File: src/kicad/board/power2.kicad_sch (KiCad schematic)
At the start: 22 parts, among them J6 PWR_EN, Q1 DMG2305UX, U2 BQ25172, U3 TLV61070A, U4 XC6206P332MR

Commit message: wip
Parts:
- C4, C5, C7, C8, C9: footprint Capacitor_SMD:C_0805_2012Metric -> Capacitor_SMD:C_0603_1608Metric; Vendor C15850 -> C19702
- C6: footprint Capacitor_SMD:C_0805_2012Metric -> Capacitor_SMD:C_0603_1608Metric; Vendor C45783 -> C59461
- R13, R15: footprint Resistor_SMD:R_0805_2012Metric -> Resistor_SMD:R_0603_1608Metric; Vendor C17530 -> C13167
- R16: footprint Resistor_SMD:R_0805_2012Metric -> Resistor_SMD:R_0603_1608Metric; Vendor C17593 -> C22967
- R17: footprint Resistor_SMD:R_0805_2012Metric -> Resistor_SMD:R_0603_1608Metric; Vendor C4328 -> C4184
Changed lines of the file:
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@@
       (effects (font (size 1.27 1.27)) (justify left))
     )
-    (property "Footprint" "Capacitor_SMD:C_0805_2012Metric" (id 2) (at 199.0852 140.97 0)
+    (property "Footprint" "Capacitor_SMD:C_0603_1608Metric" (id 2) (at 199.0852 140.97 0)
       (effects (font (size 1.27 1.27)) hide)
     )
@@
       (effects (font (size 1.27 1.27)) hide)
     )
-    (property "Vendor" "C15850" (id 4) (at 198.12 137.16 0)
+    (property "Vendor" "C19702" (id 4) (at 198.12 137.16 0)
       (effects (font (size 1.27 1.27)) hide)
     )
@@
       (effects (font (size 1.27 1.27)) (justify left))
     )
-    (property "Footprint" "Capacitor_SMD:C_0805_2012Metric" (id 2) (at 121.6152 109.22 0)
+    (property "Footprint" "Capacitor_SMD:C_0603_1608Metric" (id 2) (at 121.6152 109.22 0)
       (effects (font (size 1.27 1.27)) hide)
     )
@@
       (effects (font (size 1.27 1.27)) hide)
     )
-    (property "Vendor" "C15850" (id 4) (at 120.65 105.41 0)
+    (property "Vendor" "C19702" (id 4) (at 120.65 105.41 0)
       (effects (font (size 1.27 1.27)) hide)
     )
@@
       (effects (font (size 1.27 1.27)) (justify left))
     )
-    (property "Footprint" "Resistor_SMD:R_0805_2012Metric" (id 2) (at 159.512 66.04 90)
+    (property "Footprint" "Resistor_SMD:R_0603_1608Metric" (id 2) (at 159.512 66.04 90)
       (effects (font (size 1.27 1.27)) hide)
     )
@@
       (effects (font (size 1.27 1.27)) hide)
     )
-    (property "Vendor" "C4328" (id 4) (at 161.29 66.04 0)
+    (property "Vendor" "C4184" (id 4) (at 161.29 66.04 0)
       (effects (font (size 1.27 1.27)) hide)
     )
@@
       (effects (font (size 1.27 1.27)) (justify left))
     )
-    (property "Footprint" "Resistor_SMD:R_0805_2012Metric" (id 2) (at 151.257 133.35 90)
+    (property "Footprint" "Resistor_SMD:R_0603_1608Metric" (id 2) (at 151.257 133.35 90)
       (effects (font (size 1.27 1.27)) hide)
     )
@@
       (effects (font (size 1.27 1.27)) hide)
     )
-    (property "Vendor" "C17530" (id 4) (at 153.035 133.35 0)
+    (property "Vendor" "C13167" (id 4) (at 153.035 133.35 0)
       (effects (font (size 1.27 1.27)) hide)
     )
@@
     (property "Reference" "R13" (id 0) (at 132.08 43.18 90))
     (property "Value" "2K7" (id 1) (at 132.08 45.72 90))
-    (property "Footprint" "Resistor_SMD:R_0805_2012Metric" (id 2) (at 132.08 47.498 90)
+    (property "Footprint" "Resistor_SMD:R_0603_1608Metric" (id 2) (at 132.08 47.498 90)
       (effects (font (size 1.27 1.27)) hide)
     )
@@
       (effects (font (size 1.27 1.27)) hide)
     )
-    (property "Vendor" "C17530" (id 4) (at 132.08 45.72 0)
+    (property "Vendor" "C13167" (id 4) (at 132.08 45.72 0)
       (effects (font (size 1.27 1.27)) hide)
     )
@@
       (effects (font (size 1.27 1.27)) (justify left))
     )
-    (property "Footprint" "Capacitor_SMD:C_0805_2012Metric" (id 2) (at 169.8752 69.85 0)
+    (property "Footprint" "Capacitor_SMD:C_0603_1608Metric" (id 2) (at 169.8752 69.85 0)
       (effects (font (size 1.27 1.27)) hide)
     )
@@
       (effects (font (size 1.27 1.27)) hide)
     )
-    (property "Vendor" "C15850" (id 4) (at 168.91 66.04 0)
+    (property "Vendor" "C19702" (id 4) (at 168.91 66.04 0)
       (effects (font (size 1.27 1.27)) hide)
     )
@@
       (effects (font (size 1.27 1.27)) (justify left))
     )
-    (property "Footprint" "Capacitor_SMD:C_0805_2012Metric" (id 2) (at 176.2252 140.97 0)
+    (property "Footprint" "Capacitor_SMD:C_0603_1608Metric" (id 2) (at 176.2252 140.97 0)
       (effects (font (size 1.27 1.27)) hide)
     )
@@
       (effects (font (size 1.27 1.27)) hide)
     )
-    (property "Vendor" "C15850" (id 4) (at 175.26 137.16 0)
+    (property "Vendor" "C19702" (id 4) (at 175.26 137.16 0)
       (effects (font (size 1.27 1.27)) hide)
     )
@@
       (effects (font (size 1.27 1.27)) (justify left))
     )
-    (property "Footprint" "Resistor_SMD:R_0805_2012Metric" (id 2) (at 153.162 66.04 90)
+    (property "Footprint" "Resistor_SMD:R_0603_1608Metric" (id 2) (at 153.162 66.04 90)
       (effects (font (size 1.27 1.27)) hide)
     )
@@
       (effects (font (size 1.27 1.27)) hide)
     )
-    (property "Vendor" "C17593" (id 4) (at 154.94 66.04 0)
+    (property "Vendor" "C22967" (id 4) (at 154.94 66.04 0)
       (effects (font (size 1.27 1.27)) hide)
     )
@@
       (effects (font (size 1.27 1.27)) (justify left))
     )
-    (property "Footprint" "Capacitor_SMD:C_0805_2012Metric" (id 2) (at 108.9152 66.04 0)
+    (property "Footprint" "Capacitor_SMD:C_0603_1608Metric" (id 2) (at 108.9152 66.04 0)
       (effects (font (size 1.27 1.27)) hide)
     )
@@
       (effects (font (size 1.27 1.27)) hide)
     )
-    (property "Vendor" "C15850" (id 4) (at 107.95 62.23 0)
+    (property "Vendor" "C19702" (id 4) (at 107.95 62.23 0)
       (effects (font (size 1.27 1.27)) hide)
     )
@@
       (effects (font (size 1.27 1.27)) (justify left))
     )
-    (property "Footprint" "Capacitor_SMD:C_0805_2012Metric" (id 2) (at 164.1602 128.27 0)
+    (property "Footprint" "Capacitor_SMD:C_0603_1608Metric" (id 2) (at 164.1602 128.27 0)
       (effects (font (size 1.27 1.27)) hide)
     )
@@
       (effects (font (size 1.27 1.27)) hide)
     )
-    (property "Vendor" "C45783" (id 4) (at 163.195 124.46 0)
-      (effects (font (size 1.27 1.27)) hide)
-    )
+    (property "Vendor" "C59461" (id 4) (at 163.195 124.46 0)
+      (effects (font (size 1.27 1.27)) hide)
+    )

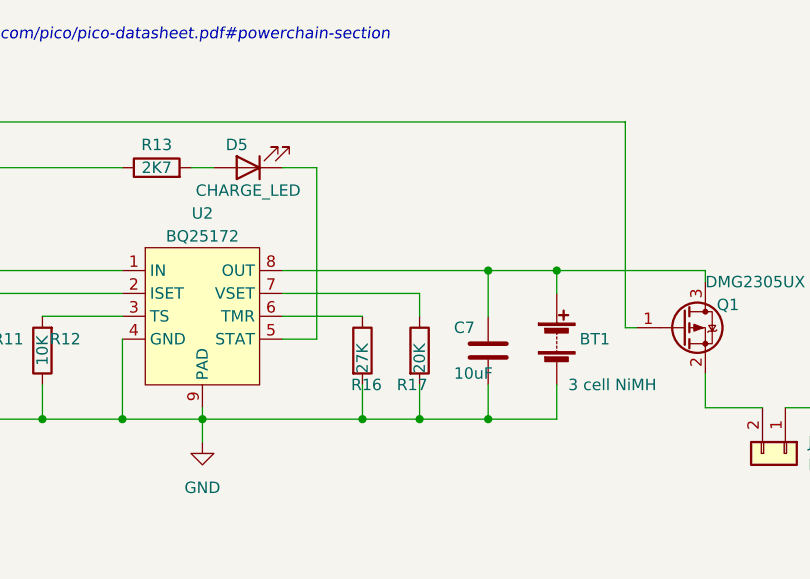
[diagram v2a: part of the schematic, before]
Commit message: update
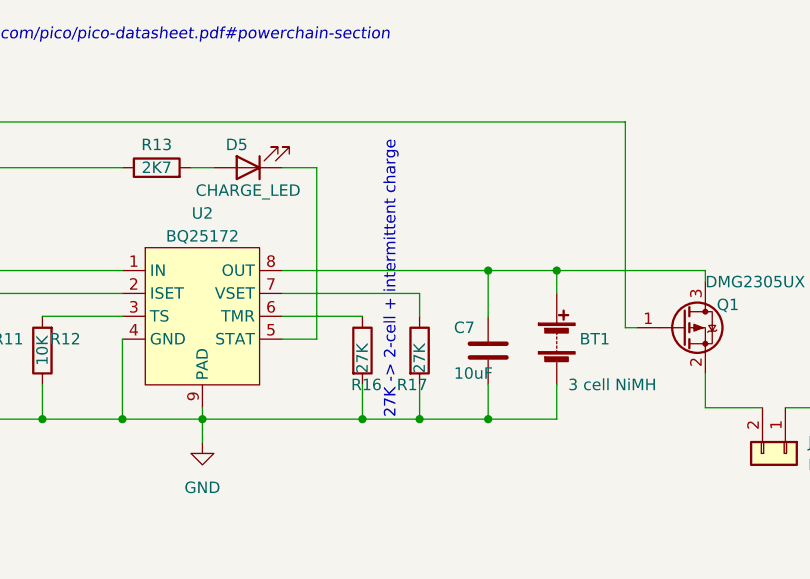
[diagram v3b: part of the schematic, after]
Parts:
- R17: value 20K -> 27K; Vendor C4184 -> C22967
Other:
- note added: "27K -> 2-cell + intermittent charge"
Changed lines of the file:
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@@
+    (effects (font (size 1.27 1.27)) (justify left bottom))
+  )
+  (text "27K -> 2-cell + intermittent charge\n" (at 158.75 73.66 90)
     (effects (font (size 1.27 1.27)) (justify left bottom))
   )
@@
       (effects (font (size 1.27 1.27)) (justify left))
     )
-    (property "Value" "20K" (id 1) (at 161.29 68.58 90)
+    (property "Value" "27K" (id 1) (at 161.29 68.58 90)
       (effects (font (size 1.27 1.27)) (justify left))
     )
@@
       (effects (font (size 1.27 1.27)) hide)
     )
-    (property "Vendor" "C4184" (id 4) (at 161.29 66.04 0)
+    (property "Vendor" "C22967" (id 4) (at 161.29 66.04 0)
       (effects (font (size 1.27 1.27)) hide)
     )
